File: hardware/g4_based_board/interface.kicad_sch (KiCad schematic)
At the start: 39 parts, among them J8 USB_C_Receptacle_USB2.0, J9 Micro_SD_Card_Det1, Q1 NPN, Q2 NPN, SW3 DOWN, SW7 UP, SW8 ENTER, SW9 WAKE

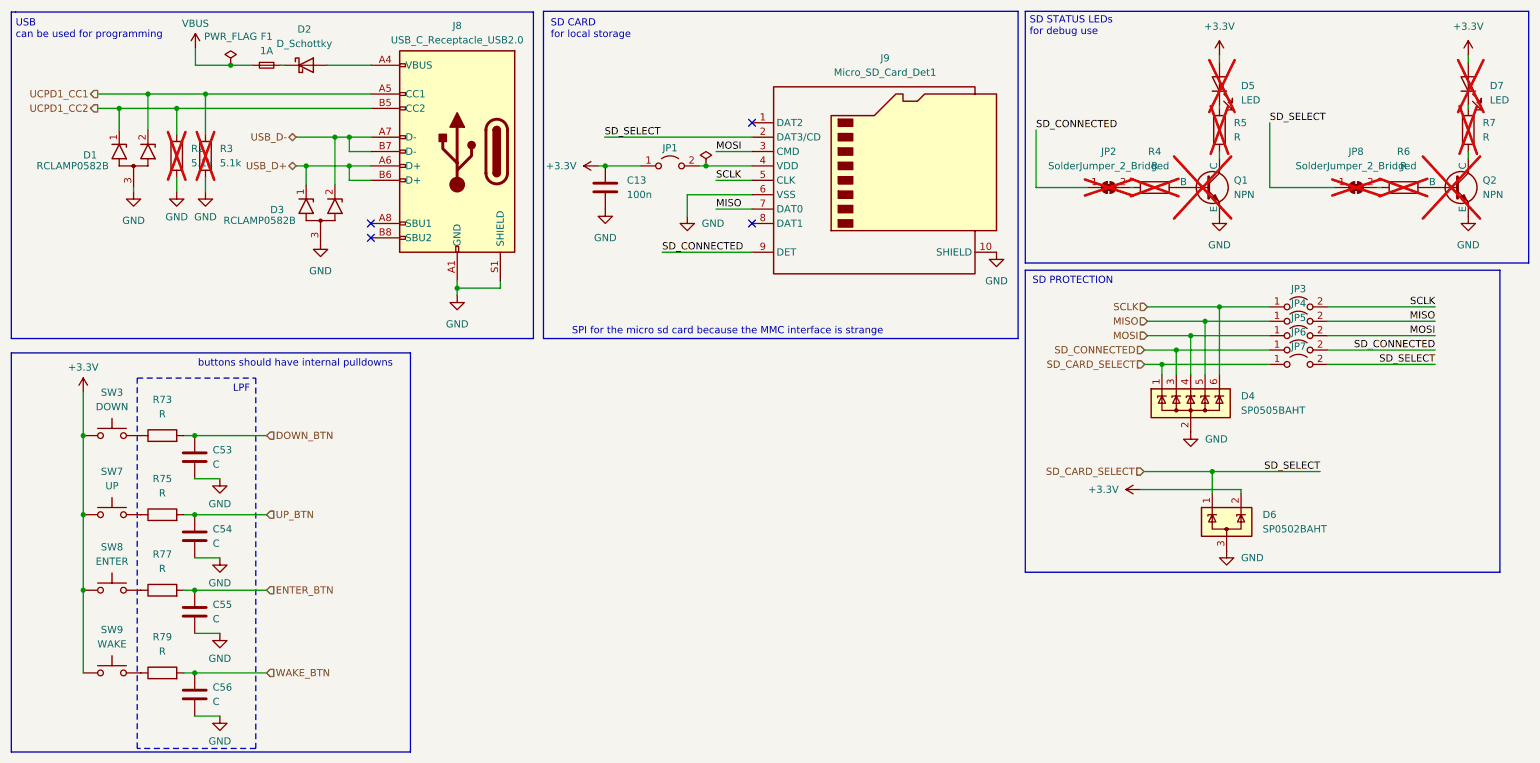
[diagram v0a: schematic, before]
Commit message: rev-1
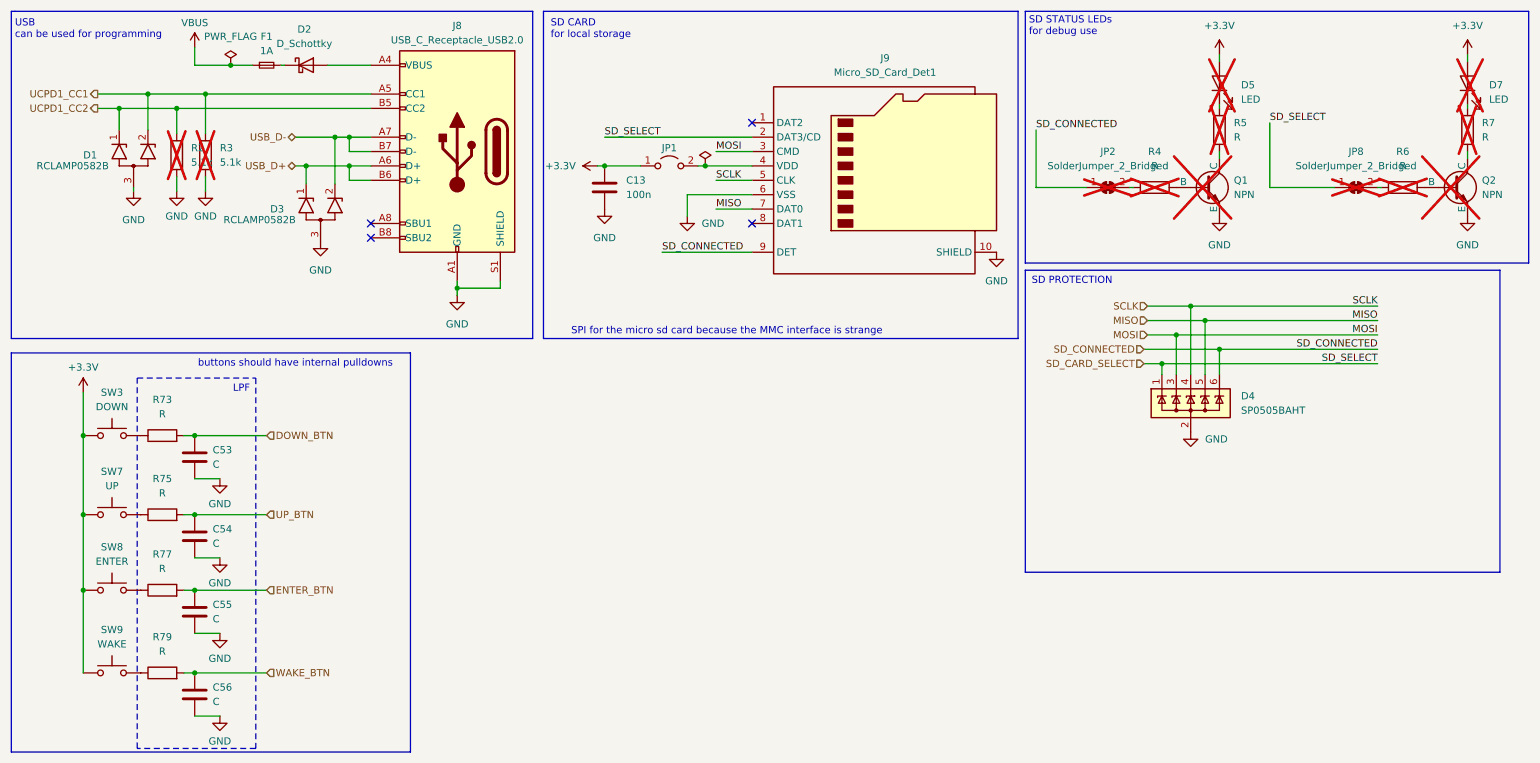
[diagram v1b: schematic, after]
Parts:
- removed D6: SP0502BAHT, Package_TO_SOT_SMD:SOT-23, symbol Power_Protection:SP0502BAHT
- removed JP3, JP4, JP5, JP6, JP7: Jumper_2_Open, Jumper:SolderJumper-2_P1.3mm_Open_TrianglePad1.0x1.5mm, symbol Jumper:Jumper_2_Open
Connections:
- net MOSI: now also D4.3 (K); no longer D4.4 (K)
- net SCLK: now also D4.4 (K); no longer D4.6 (K)
- net SD_CONNECTED: now also D4.6 (K); no longer D4.3 (K)
